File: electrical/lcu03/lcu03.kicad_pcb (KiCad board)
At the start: 2 copper layers, 99.5 x 50 mm, 121 parts, among them P1 screw, P10 swd, P11 stepper_conn, P12 stepper_conn, P13 stepper_conn, P14 stepper_conn, P15 stepper_conn, P16 screw, P17 screw, P2 screw, P3 screw, P4 screw, P5 ext-1, P6 ~rst~, P7 mode, P8 ext-2, P9 USB_B, Q1 bc857, Q2 bc847, Q3 bc857, Q4 ntd18n06l, U1 crystal-4pin, U10 MCP1703T-3302E/CB, U2 CP2102, U3 m24c02, U4 NCP3063, U5 my-NCP1117ST50T3G, U6 ts881, U7 lb1930mc, U8 a4985, U9 a4985

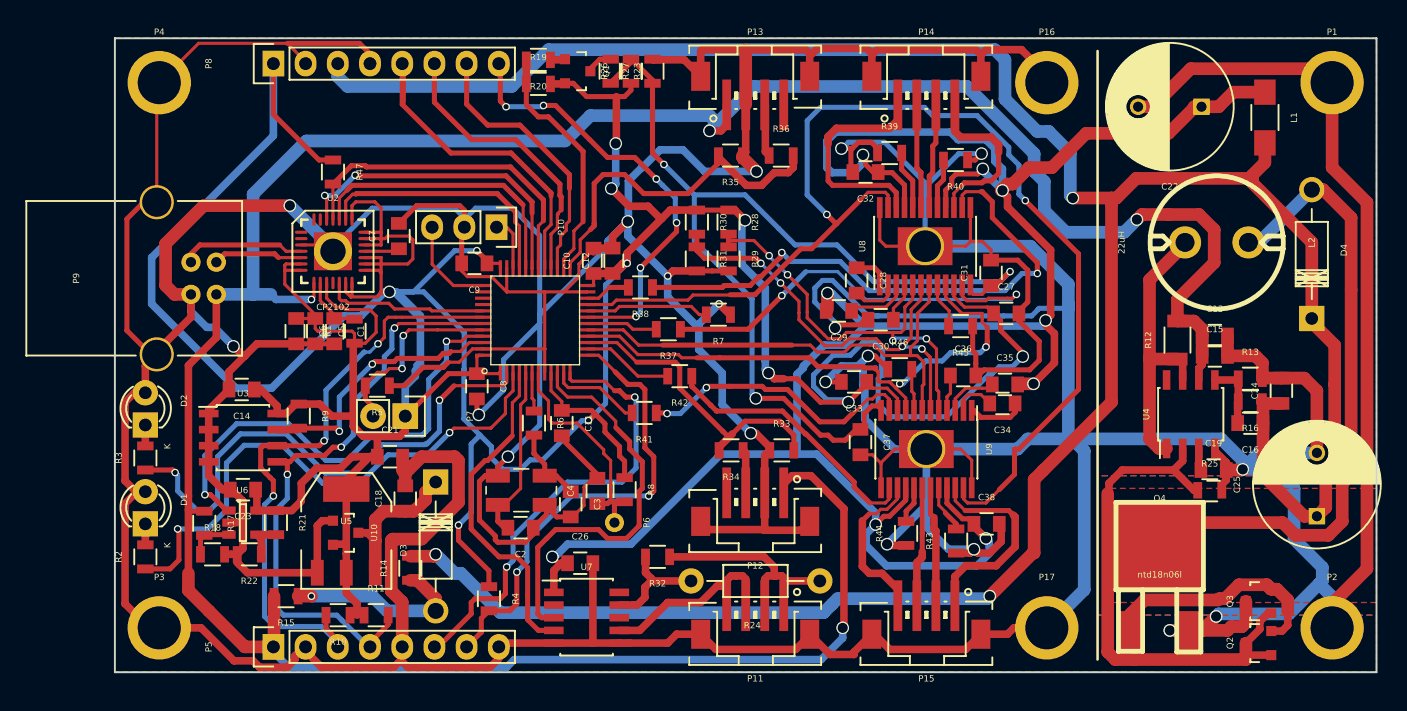
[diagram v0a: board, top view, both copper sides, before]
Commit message: Finished beautifications. Generated gerber files.
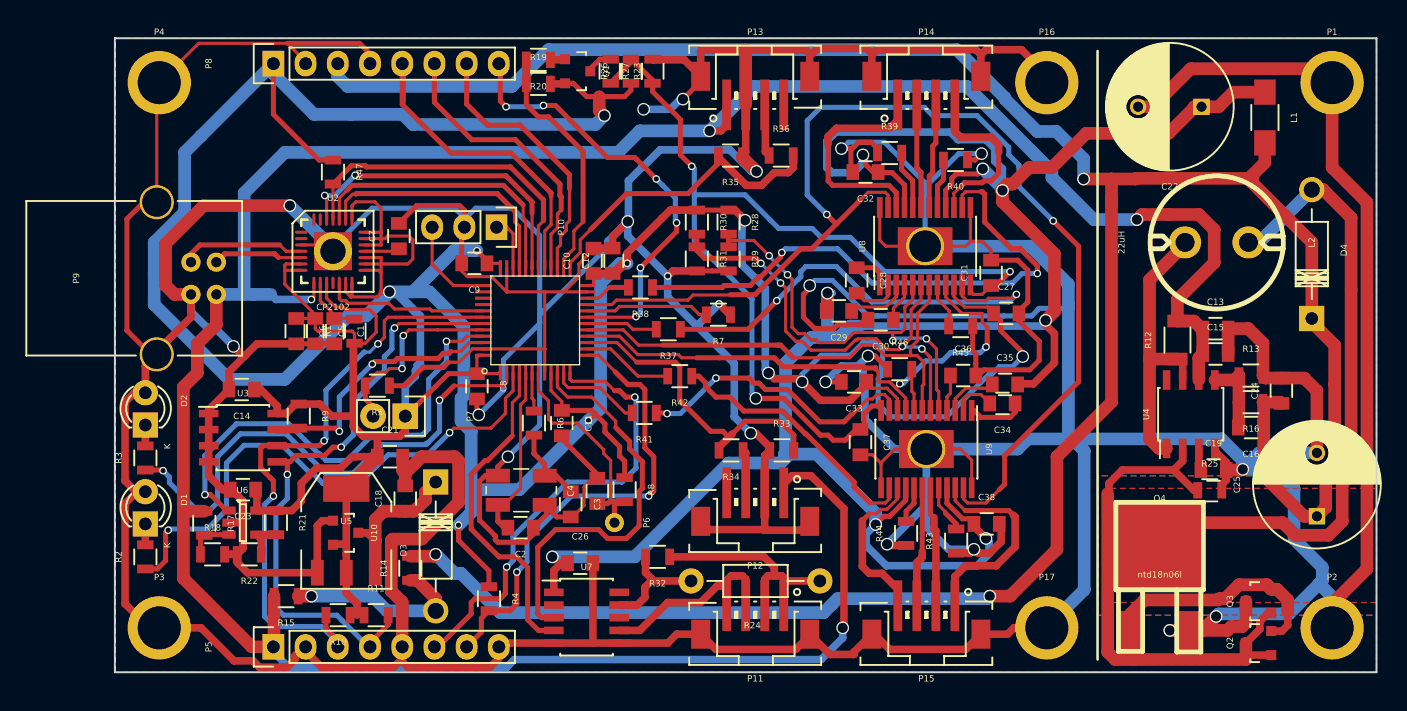
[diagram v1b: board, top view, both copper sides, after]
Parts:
- moved C13 0.55 mm to (174.8, 93.9)
- moved C16 0.35 mm to (177.6, 101.7)
- moved R13 0.25 mm to (177.6, 97.6)
- moved C15 0.16 mm to (174.8, 95.9)
- moved R16 0.07 mm to (177.6, 99.7)
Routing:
- net VDD: track 381.9 -> 406.5 mm, vias 11 -> 10
- net GND: track 859.7 -> 869.6 mm, vias 19 -> 21
- net /Vbus: track 228.8 -> 223.6 mm
- net /stepper-subcircuit-1/Vbb: track 177.3 -> 180.9 mm, vias 9 -> 8
- net /reg-fb: track 215.4 -> 212.0 mm
- net /hall2: track 28.6 -> 25.4 mm
- net /stepper-subcircuit-1/ms2: track 34.4 -> 35.8 mm
- net /stepper-subcircuit-1/ms1: track 32.7 -> 34.1 mm
- net Net-(R37-Pad1): track 35.0 -> 36.1 mm
- net Net-(C16-Pad2): track 5.41 -> 6.23 mm
- net /stepper-subcircuit-1/ref: track 80.7 -> 80.0 mm
- net Net-(R41-Pad1): track 22.4 -> 23.0 mm
- net /hall1: track 24.1 -> 24.6 mm
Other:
- board text removed: "Here use 2n4 instead to decrease frequency down to 150kHz."
